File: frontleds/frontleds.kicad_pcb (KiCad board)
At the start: 2 copper layers, 30 x 21.8 mm, 8 parts, among them J1 Conn_01x04, J2 Conn_01x04

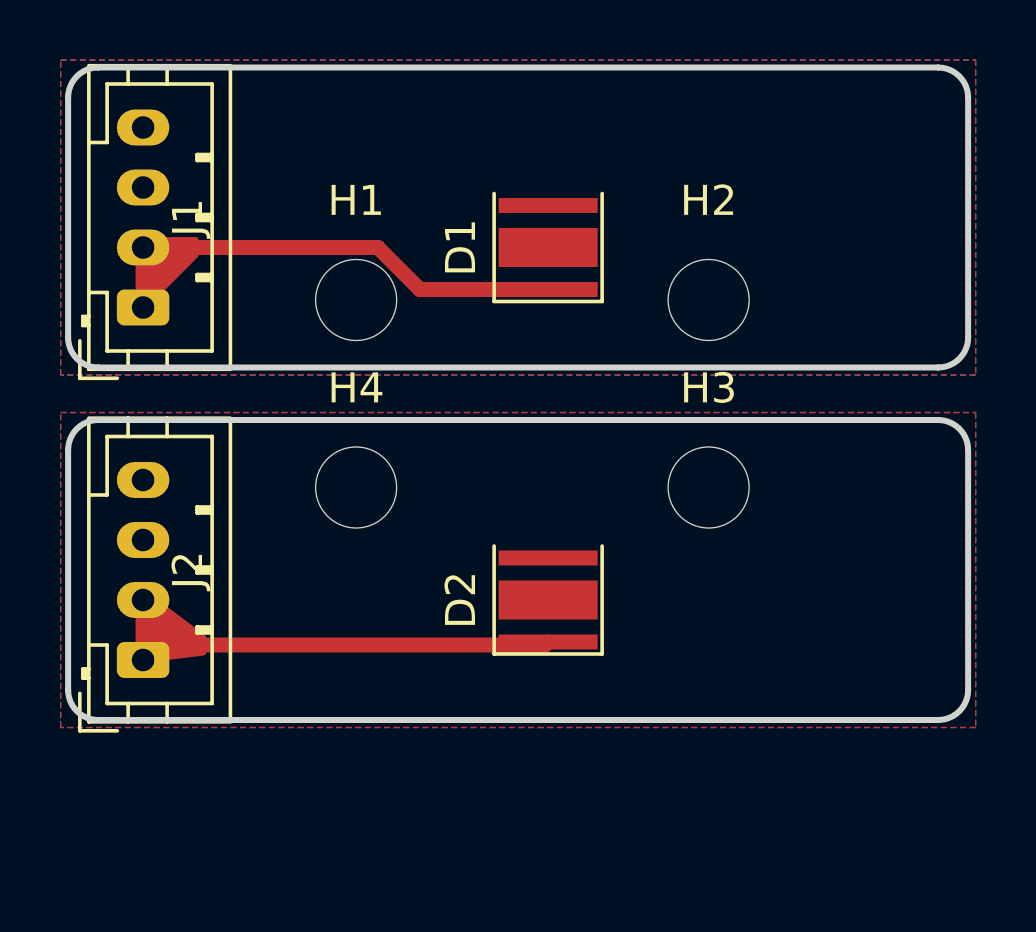
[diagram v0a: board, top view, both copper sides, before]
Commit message: smol boi
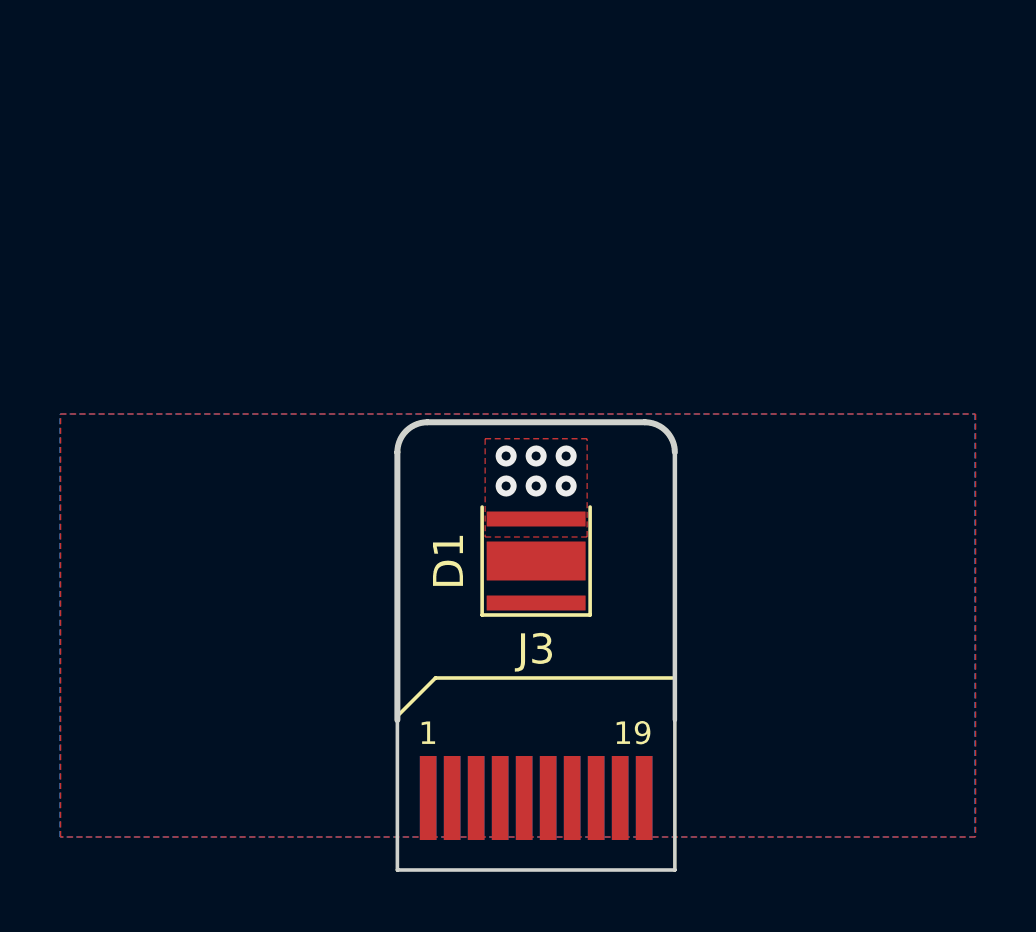
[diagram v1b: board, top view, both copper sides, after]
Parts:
- removed D2: LED_Pad, LED_SMD:LED_Cree-XP-GWT
- removed H1, H2, H3, H4: MountingHole, MountingHole:MountingHole_2.7mm_M2.5_DIN965
- removed J1, J2: Conn_01x04, Connector_JST:JST_PH_B4B-PH-K_1x04_P2.00mm_Vertical
- added J3: Conn_02x10_Odd_Even, Connector_Samtec_HSEC8:Samtec_HSEC8-110-X-X-DV_2x10_P0.8mm_Edge, F.Cu at (165.6, 84.0)
- moved D1 10.5 mm to (165.6, 73.7)
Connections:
- D1 pad 1: /PWR1 -> GND
- D1 pad 2: /GND1 -> /PWR1
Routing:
- net /PWR1: track 16.6 -> 0.00 mm, vias 0 -> 6
- net /PWR2: track 16.2 -> 0.00 mm
- added copper zone on B.Cu, net /PWR1
- added copper zone on F.Cu, net /PWR1
- added copper zone on F.Cu, net GND
- removed copper zone on B.Cu, net /GND1
- removed copper zone on F.Cu, net /GND1
- removed copper zone on B.Cu, net /GND2
- removed copper zone on F.Cu, net /GND2
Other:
- board size 30 x 21.8 mm -> 9.2 x 9.9 mm

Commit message: changed front leds to use dedicated led current drivers
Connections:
- D1 pad 3: unconnected-(D1-PAD-Pad3) -> GND
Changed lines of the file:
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@@
 	)
 	(net 0 "")
-	(net 1 "unconnected-(D1-PAD-Pad3)")
-	(net 2 "/PWR1")
-	(net 3 "GND")
+	(net 1 "/PWR1")
+	(net 2 "GND")
 	(footprint "Connector_Samtec_HSEC8:Samtec_HSEC8-110-X-X-DV_2x10_P0.8mm_Edge"
 		(layer "F.Cu")
@@
 			(size 0.55 2.8)
 			(layers "F.Cu" "F.Mask")
-			(net 3 "GND")
+			(net 2 "GND")
 			(pinfunction "Pin_1")
 			(pintype "passive")
@@
 			(size 0.55 2.8)
 			(layers "B.Cu" "B.Mask")
-			(net 2 "/PWR1")
+			(net 1 "/PWR1")
 			(pinfunction "Pin_2")
 			(pintype "passive")
@@
 			(size 0.55 2.8)
 			(layers "F.Cu" "F.Mask")
-			(net 3 "GND")
+			(net 2 "GND")
 			(pinfunction "Pin_3")
 			(pintype "passive")
@@
 			(size 0.55 2.8)
 			(layers "B.Cu" "B.Mask")
-			(net 2 "/PWR1")
+			(net 1 "/PWR1")
 			(pinfunction "Pin_4")
 			(pintype "passive")
@@
 			(size 0.55 2.8)
 			(layers "F.Cu" "F.Mask")
-			(net 3 "GND")
+			(net 2 "GND")
 			(pinfunction "Pin_5")
 			(pintype "passive")
@@
 			(size 0.55 2.8)
 			(layers "B.Cu" "B.Mask")
-			(net 2 "/PWR1")
+			(net 1 "/PWR1")
 			(pinfunction "Pin_6")
 			(pintype "passive")
@@
 			(size 0.55 2.8)
 			(layers "F.Cu" "F.Mask")
-			(net 3 "GND")
+			(net 2 "GND")
 			(pinfunction "Pin_7")
 			(pintype "passive")
@@
 			(size 0.55 2.8)
 			(layers "B.Cu" "B.Mask")
-			(net 2 "/PWR1")
+			(net 1 "/PWR1")
 			(pinfunction "Pin_8")
 			(pintype "passive")
@@
 			(size 0.55 2.8)
 			(layers "F.Cu" "F.Mask")
-			(net 3 "GND")
+			(net 2 "GND")
 			(pinfunction "Pin_9")
 			(pintype "passive")
@@
 			(size 0.55 2.8)
 			(layers "B.Cu" "B.Mask")
-			(net 2 "/PWR1")
+			(net 1 "/PWR1")
 			(pinfunction "Pin_10")
 			(pintype "passive")
@@
 			(size 0.55 2.8)
 			(layers "F.Cu" "F.Mask")
-			(net 3 "GND")
+			(net 2 "GND")
 			(pinfunction "Pin_11")
 			(pintype "passive")
@@
 			(size 0.55 2.8)
 			(layers "B.Cu" "B.Mask")
-			(net 2 "/PWR1")
+			(net 1 "/PWR1")
 			(pinfunction "Pin_12")
 			(pintype "passive")
@@
 			(size 0.55 2.8)
 			(layers "F.Cu" "F.Mask")
-			(net 3 "GND")
+			(net 2 "GND")
 			(pinfunction "Pin_13")
 			(pintype "passive")
@@
 			(size 0.55 2.8)
 			(layers "B.Cu" "B.Mask")
-			(net 2 "/PWR1")
+			(net 1 "/PWR1")
 			(pinfunction "Pin_14")
 			(pintype "passive")
@@
 			(size 0.55 2.8)
 			(layers "F.Cu" "F.Mask")
-			(net 3 "GND")
+			(net 2 "GND")
 			(pinfunction "Pin_15")
 			(pintype "passive")
@@
 			(size 0.55 2.8)
 			(layers "B.Cu" "B.Mask")
-			(net 2 "/PWR1")
+			(net 1 "/PWR1")
 			(pinfunction "Pin_16")
 			(pintype "passive")
@@
 			(size 0.55 2.8)
 			(layers "F.Cu" "F.Mask")
-			(net 3 "GND")
+			(net 2 "GND")
 			(pinfunction "Pin_17")
 			(pintype "passive")
@@
 			(size 0.55 2.8)
 			(layers "B.Cu" "B.Mask")
-			(net 2 "/PWR1")
+			(net 1 "/PWR1")
 			(pinfunction "Pin_18")
 			(pintype "passive")
@@
 			(size 0.55 2.8)
 			(layers "F.Cu" "F.Mask")
-			(net 3 "GND")
+			(net 2 "GND")
 			(pinfunction "Pin_19")
 			(pintype "passive")
@@
 			(size 0.55 2.8)
 			(layers "B.Cu" "B.Mask")
-			(net 2 "/PWR1")
+			(net 1 "/PWR1")
 			(pinfunction "Pin_20")
 			(pintype "passive")
@@
 			(size 0.5 3.3)
 			(layers "F.Cu" "F.Mask" "F.Paste")
-			(net 3 "GND")
+			(net 2 "GND")
 			(pinfunction "K")
 			(pintype "passive")
@@
 			(size 0.5 3.3)
 			(layers "F.Cu" "F.Mask" "F.Paste")
-			(net 2 "/PWR1")
+			(net 1 "/PWR1")
 			(pinfunction "A")
 			(pintype "passive")
@@
 			(size 1.3 3.3)
 			(layers "F.Cu" "F.Mask")
-			(net 1 "unconnected-(D1-PAD-Pad3)")
+			(net 2 "GND")
 			(pinfunction "PAD")
-			(pintype "passive+no_connect")
+			(pintype "passive")
 		)
 		(embedded_fonts no)
@@
 		(layers "F.Cu" "B.Cu")
 		(free yes)
-		(net 2)
+		(net 1)
 	)
 	(via
@@
 		(layers "F.Cu" "B.Cu")
 		(free yes)
-		(net 2)
+		(net 1)
 	)
 	(via
@@
 		(layers "F.Cu" "B.Cu")
 		(free yes)
-		(net 2)
+		(net 1)
 	)
 	(via
@@
 		(layers "F.Cu" "B.Cu")
 		(free yes)
-		(net 2)
+		(net 1)
 	)
 	(via
@@
 		(layers "F.Cu" "B.Cu")
 		(free yes)
-		(net 2)
+		(net 1)
 	)
 	(via
@@
 		(layers "F.Cu" "B.Cu")
 		(free yes)
+		(net 1)
+	)
+	(zone
 		(net 2)
-	)
-	(zone
-		(net 3)
 		(net_name "GND")
 		(layer "F.Cu")
@@
 	)
 	(zone
-		(net 2)
+		(net 1)
 		(net_name "/PWR1")
 		(layer "F.Cu")
@@
 	)
 	(zone
-		(net 2)
+		(net 1)
 		(net_name "/PWR1")
 		(layer "B.Cu")

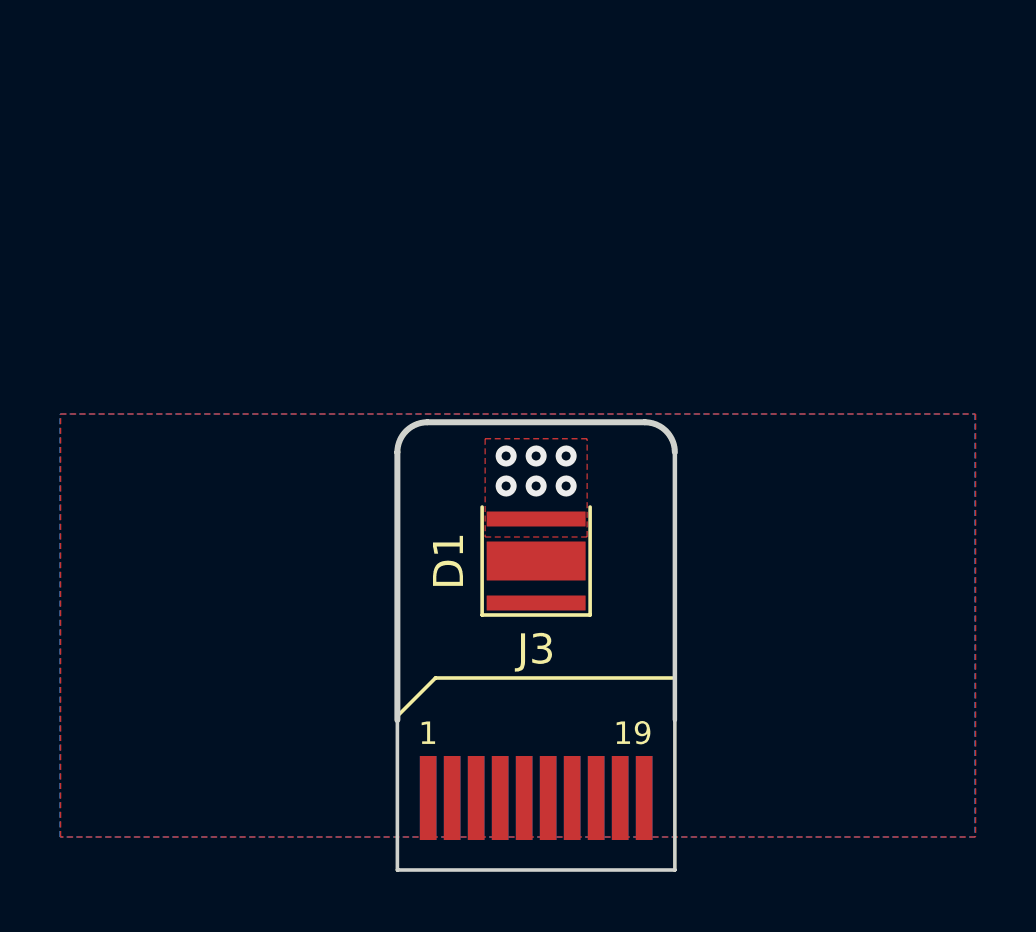
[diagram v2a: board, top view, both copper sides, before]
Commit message: export steps
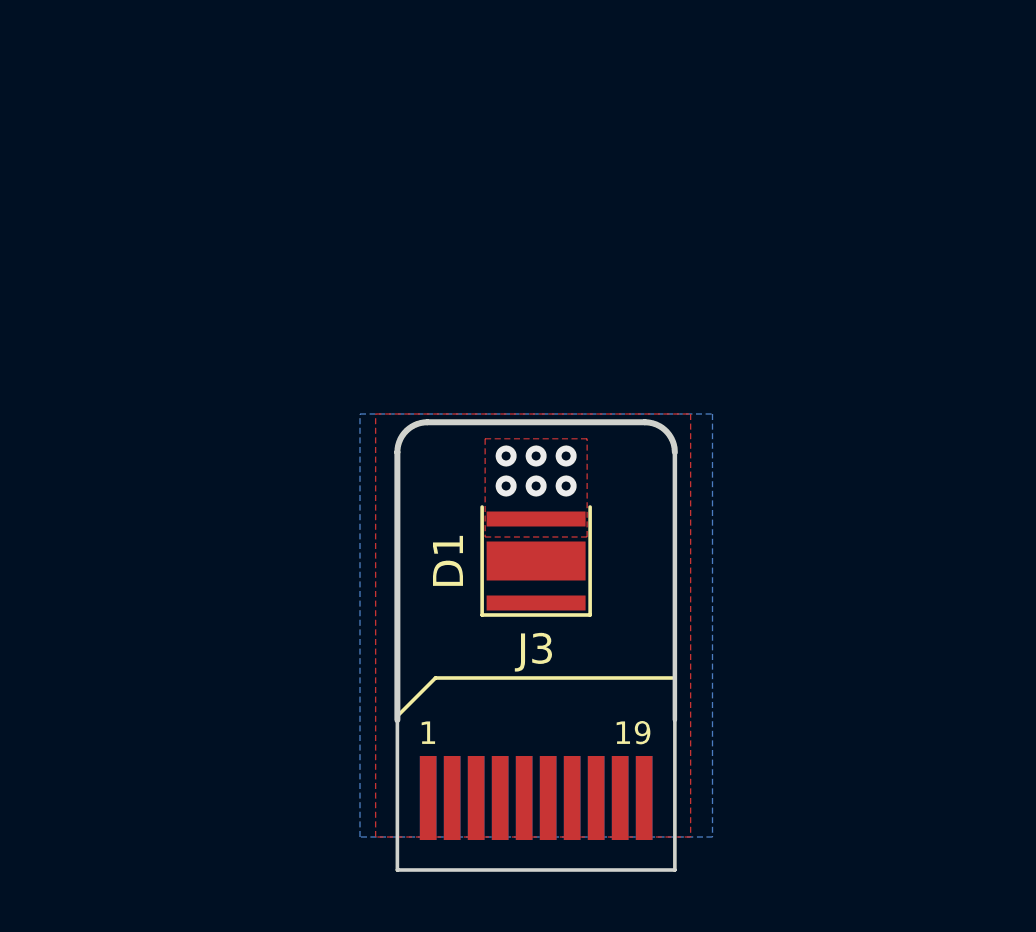
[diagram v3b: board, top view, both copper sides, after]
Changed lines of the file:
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@@
 		(polygon
 			(pts
-				(xy 149.75 82.9) (xy 149.75 68.8) (xy 180.25 68.8) (xy 180.25 82.9)
+				(xy 160.25 82.9) (xy 160.25 68.8) (xy 170.75 68.8) (xy 170.75 82.9)
 			)
 		)
@@
 		(polygon
 			(pts
-				(xy 149.729068 82.9) (xy 149.729068 68.8) (xy 180.229068 68.8) (xy 180.229068 82.9)
+				(xy 159.729068 82.9) (xy 159.729068 68.8) (xy 171.479068 68.8) (xy 171.479068 82.9)
 			)
 		)
